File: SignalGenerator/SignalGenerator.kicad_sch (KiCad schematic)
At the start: 54 parts, among them J1 Buss PD, J2 AVR-ICSP, J3 I2C Display, J4 Conn_Coaxial, SW1 SW_Push_SPDT, T1 Transformer_1P_SS, U1 LM7805_TO220, U2 ATmega328P-AU, U3 LM7812_TO220, U4 LM7912_TO220, U5 AD8021, U6 AD9833BRMZ, X1 Oscillator, Y1 Crystal_cfpx-104

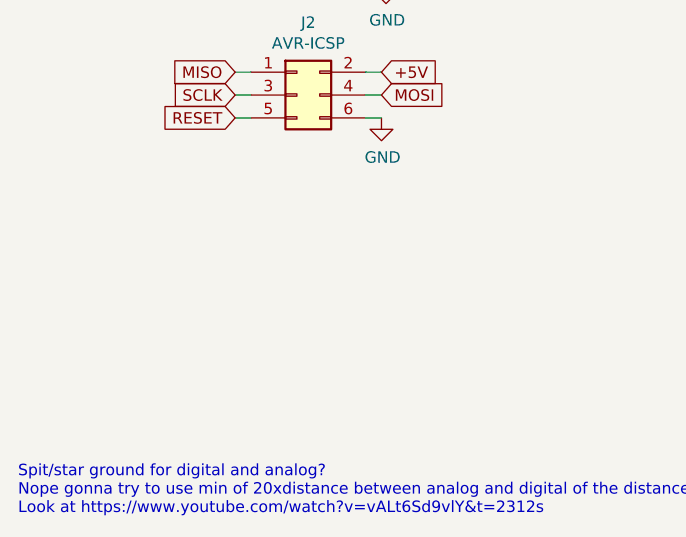
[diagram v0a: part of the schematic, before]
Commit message: made some stuff again
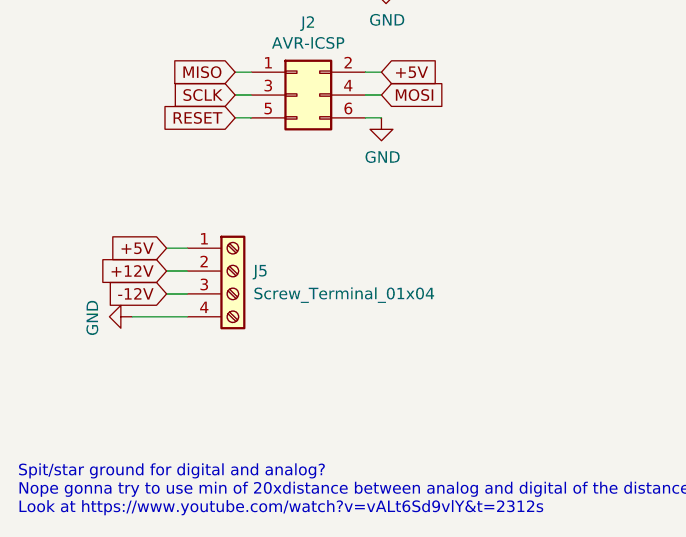
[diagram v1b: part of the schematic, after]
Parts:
- added J5: Screw_Terminal_01x04, TerminalBlock_Altech:Altech_AK300_1x04_P5.00mm_45-Degree, symbol Connector:Screw_Terminal_01x04
- SW1: footprint Connector_PinHeader_2.54mm:PinHeader_1x03_P2.54mm_Vertical_SMD_Pin1Left -> Connector_PinHeader_2.54mm:PinHeader_1x03_P2.54mm_Vertical
- Y1: footprint Crystal:Crystal_SMD_5032-2Pin_5.0x3.2mm_HandSoldering -> Crystal:Crystal_SMD_5032-4Pin_5.0x3.2mm Handsolder
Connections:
- net +12V: now also J5.2 (Pin_2)
- net +5V: now also J5.1 (Pin_1)
- net -12V: now also J5.3 (Pin_3)
- net GND: now also J5.4 (Pin_4)
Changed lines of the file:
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@@
+    (stroke (width 0) (type default) (color 0 0 0 0))
+  )
+  (wire (pts (xy 28.194 171.45) (xy 34.29 171.45))
     (stroke (width 0) (type default) (color 0 0 0 0))
   )
@@
     (stroke (width 0) (type default) (color 0 0 0 0))
   )
+  (wire (pts (xy 32.004 163.83) (xy 34.29 163.83))
+    (stroke (width 0) (type default) (color 0 0 0 0))
+  )
   (wire (pts (xy 165.1 72.39) (xy 165.1 69.85))
     (stroke (width 0) (type default) (color 0 0 0 0))
@@
     (stroke (width 0) (type default) (color 0 0 0 0))
   )
+  (wire (pts (xy 32.004 168.91) (xy 34.29 168.91))
+    (stroke (width 0) (type default) (color 0 0 0 0))
+  )
   (wire (pts (xy 181.356 118.872) (xy 184.15 118.872))
     (stroke (width 0) (type default) (color 0 0 0 0))
@@
   )
   (wire (pts (xy 151.765 34.29) (xy 137.795 34.29))
+    (stroke (width 0) (type default) (color 0 0 0 0))
+  )
+  (wire (pts (xy 32.004 166.37) (xy 34.29 166.37))
     (stroke (width 0) (type default) (color 0 0 0 0))
   )
@@
     )
   )
+  (global_label "+12V" (shape input) (at 32.004 166.37 180) (fields_autoplaced)
+    (effects (font (size 1.27 1.27)) (justify right))
+    (property "Intersheet References" "${INTERSHEET_REFS}" (id 0) (at 192.024 189.23 0)
+      (effects (font (size 1.27 1.27)) hide)
+    )
+  )
   (global_label "PD4" (shape input) (at 39.37 129.032 180) (fields_autoplaced)
     (effects (font (size 1.27 1.27)) (justify right))
@@
     )
   )
+  (global_label "+5V" (shape input) (at 32.004 163.83 180) (fields_autoplaced)
+    (effects (font (size 1.27 1.27)) (justify right))
+    (property "Intersheet References" "${INTERSHEET_REFS}" (id 0) (at 88.392 296.164 0)
+      (effects (font (size 1.27 1.27)) hide)
+    )
+  )
   (global_label "+5V" (shape input) (at 48.26 86.614 90) (fields_autoplaced)
     (effects (font (size 1.27 1.27)) (justify left))
@@
     (effects (font (size 1.27 1.27)) (justify left))
     (property "Intersheet References" "${INTERSHEET_REFS}" (id 0) (at 0 0 0)
+      (effects (font (size 1.27 1.27)) hide)
+    )
+  )
+  (global_label "-12V" (shape input) (at 32.004 168.91 180) (fields_autoplaced)
+    (effects (font (size 1.27 1.27)) (justify right))
+    (property "Intersheet References" "${INTERSHEET_REFS}" (id 0) (at 192.659 215.9 0)
       (effects (font (size 1.27 1.27)) hide)
     )
@@
     (property "Reference" "SW1" (id 0) (at 198.12 33.909 0))
     (property "Value" "SW_Push_SPDT" (id 1) (at 198.12 31.5976 0))
-    (property "Footprint" "Connector_PinHeader_2.54mm:PinHeader_1x03_P2.54mm_Vertical_SMD_Pin1Left" (id 2) (at 198.12 26.67 0)
+    (property "Footprint" "Connector_PinHeader_2.54mm:PinHeader_1x03_P2.54mm_Vertical" (id 2) (at 198.12 26.67 0)
       (effects (font (size 1.27 1.27)) hide)
     )
@@
     (property "Reference" "Y1" (id 0) (at 181.61 66.2686 0))
     (property "Value" "Crystal_cfpx-104" (id 1) (at 156.718 65.532 0))
-    (property "Footprint" "Crystal:Crystal_SMD_5032-2Pin_5.0x3.2mm_HandSoldering" (id 2) (at 171.196 69.85 0)
+    (property "Footprint" "Crystal:Crystal_SMD_5032-4Pin_5.0x3.2mm Handsolder" (id 2) (at 171.196 69.85 0)
       (effects (font (size 1.27 1.27)) hide)
     )
@@
     (pin "2")
   )
+  (symbol (lib_id "Connector:Screw_Terminal_01x04") (at 39.37 166.37 0) (unit 1)
+    (in_bom yes) (on_board yes) (fields_autoplaced)
+    (property "Reference" "J5" (id 0) (at 41.656 166.3699 0)
+      (effects (font (size 1.27 1.27)) (justify left))
+    )
+    (property "Value" "Screw_Terminal_01x04" (id 1) (at 41.656 168.9099 0)
+      (effects (font (size 1.27 1.27)) (justify left))
+    )
+    (property "Footprint" "TerminalBlock_Altech:Altech_AK300_1x04_P5.00mm_45-Degree" (id 2) (at 39.37 166.37 0)
+      (effects (font (size 1.27 1.27)) hide)
+    )
+    (property "Datasheet" "~" (id 3) (at 39.37 166.37 0)
+      (effects (font (size 1.27 1.27)) hide)
+    )
+    (pin "1")
+    (pin "2")
+    (pin "3")
+    (pin "4")
+  )
   (symbol (lib_id "power:GND") (at 139.446 144.018 0) (unit 1)
     (in_bom yes) (on_board yes)
@@
     )
     (property "Datasheet" "" (id 3) (at 139.446 144.018 0)
+      (effects (font (size 1.27 1.27)) hide)
+    )
+    (pin "1")
+  )
+  (symbol (lib_id "power:GND") (at 28.194 171.45 270) (unit 1)
+    (in_bom yes) (on_board yes)
+    (property "Reference" "#PWR031" (id 0) (at 21.844 171.45 0)
+      (effects (font (size 1.27 1.27)) hide)
+    )
+    (property "Value" "GND" (id 1) (at 23.7998 171.577 0))
+    (property "Footprint" "" (id 2) (at 28.194 171.45 0)
+      (effects (font (size 1.27 1.27)) hide)
+    )
+    (property "Datasheet" "" (id 3) (at 28.194 171.45 0)
       (effects (font (size 1.27 1.27)) hide)
     )
@@
       (reference "#PWR030") (unit 1) (value "GND") (footprint "")
     )
+    (path "/d84d87ba-d54b-4a23-9048-632c7da722ac"
+      (reference "#PWR031") (unit 1) (value "GND") (footprint "")
+    )
     (path "/55a61499-54e1-46d6-bb9e-fac0b5ad41bb"
       (reference "#PWR0101") (unit 1) (value "GND") (footprint "")
@@
       (reference "J4") (unit 1) (value "Conn_Coaxial") (footprint "Connector_PinHeader_2.54mm:PinHeader_1x02_P2.54mm_Vertical")
     )
+    (path "/c7f8cef4-db64-4b14-ba6a-2de4c4c1cf7c"
+      (reference "J5") (unit 1) (value "Screw_Terminal_01x04") (footprint "TerminalBlock_Altech:Altech_AK300_1x04_P5.00mm_45-Degree")
+    )
     (path "/00000000-0000-0000-0000-0000620159fb"
       (reference "R1") (unit 1) (value "4.7k") (footprint "Resistor_SMD:R_0805_2012Metric_Pad1.20x1.40mm_HandSolder")
@@
     )
     (path "/00000000-0000-0000-0000-0000618b491b"
-      (reference "SW1") (unit 1) (value "SW_Push_SPDT") (footprint "Connector_PinHeader_2.54mm:PinHeader_1x03_P2.54mm_Vertical_SMD_Pin1Left")
+      (reference "SW1") (unit 1) (value "SW_Push_SPDT") (footprint "Connector_PinHeader_2.54mm:PinHeader_1x03_P2.54mm_Vertical")
     )
     (path "/00000000-0000-0000-0000-0000616b094b"
@@
     )
     (path "/71032dfc-29f3-405c-8a4d-da3fa04dca22"
-      (reference "Y1") (unit 1) (value "Crystal_cfpx-104") (footprint "Crystal:Crystal_SMD_5032-2Pin_5.0x3.2mm_HandSoldering")
-    )
-  )
+      (reference "Y1") (unit 1) (value "Crystal_cfpx-104") (footprint "Crystal:Crystal_SMD_5032-4Pin_5.0x3.2mm Handsolder")
+    )
+  )
